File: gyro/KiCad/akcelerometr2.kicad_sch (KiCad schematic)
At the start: 5 parts, among them J2 Conn_01x04_Pin, J3 Conn_01x04_Pin, J4 Conn_01x08_Pin

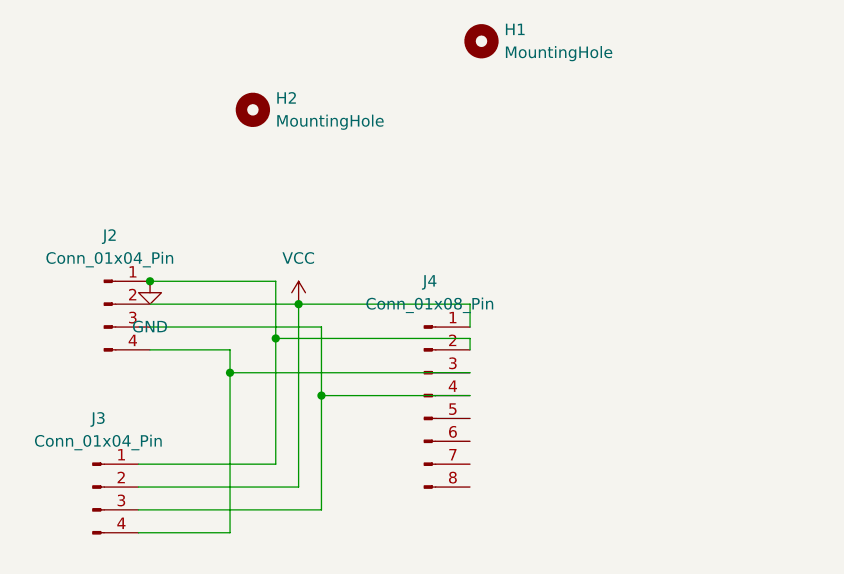
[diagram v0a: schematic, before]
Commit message: Deployed 0144617 with MkDocs version: 1.6.0
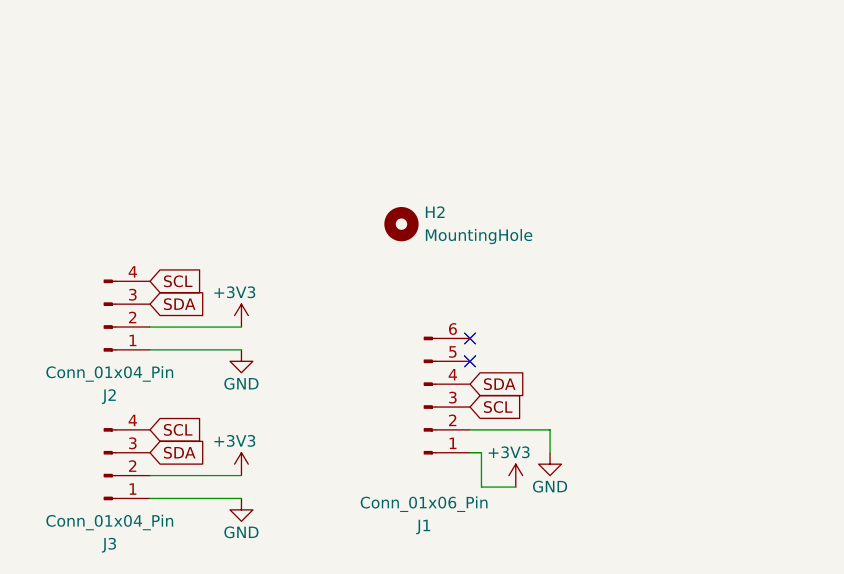
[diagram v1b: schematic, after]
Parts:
- removed H1: MountingHole, MountingHole:MountingHole_3.2mm_M3, symbol Mechanical:MountingHole
- removed J4: Conn_01x08_Pin, Connector_PinHeader_2.54mm:PinHeader_1x08_P2.54mm_Vertical, symbol Connector:Conn_01x08_Pin
- added J1: Conn_01x06_Pin, Connector_PinHeader_2.54mm:PinHeader_1x06_P2.54mm_Horizontal, symbol Connector:Conn_01x06_Pin
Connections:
- net GND: now also J1.2 (Pin_2)
- net SDA: now reaches J2.3 (Pin_3), J3.3 (Pin_3)
- net SDA: now also J1.4 (Pin_4)
- net SCL: now reaches J2.4 (Pin_4), J3.4 (Pin_4)
- net SCL: now also J1.3 (Pin_3)
- net VCC renamed +3V3
- net +3V3: now also J1.1 (Pin_1)
- no-connect marks 0 -> 2
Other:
- moved on the sheet: H2, J3

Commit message: Deployed ba208f9 with MkDocs version: 1.6.0
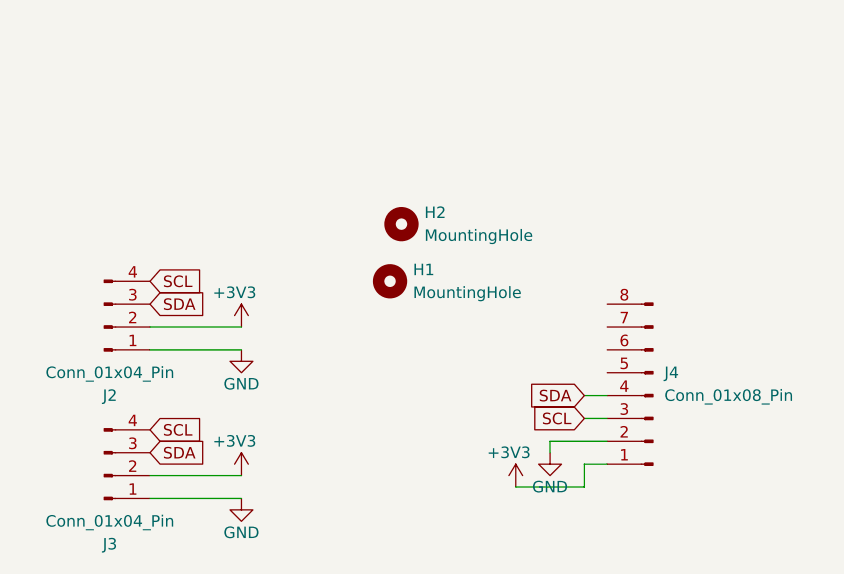
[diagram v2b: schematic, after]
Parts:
- removed J1: Conn_01x06_Pin, Connector_PinHeader_2.54mm:PinHeader_1x06_P2.54mm_Horizontal, symbol Connector:Conn_01x06_Pin
- added H1: MountingHole, MountingHole:MountingHole_3.2mm_M3, symbol Mechanical:MountingHole
- added J4: Conn_01x08_Pin, Connector_PinHeader_2.54mm:PinHeader_1x08_P2.54mm_Horizontal, symbol Connector:Conn_01x08_Pin
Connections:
- net +3V3: now also J4.1 (Pin_1)
- net GND: now also J4.2 (Pin_2)
- net SCL: now also J4.3 (Pin_3)
- net SDA: now also J4.4 (Pin_4)
- no-connect marks 2 -> 0
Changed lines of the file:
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@@
 	(generator_version "9.0")
 	(paper "A4")
-	(no_connect
-		(at 152.4 72.39)
-	)
-	(no_connect
-		(at 152.4 69.85)
-	)
 	(wire
 		(pts
@@
 	(wire
 		(pts
-			(xy 153.67 86.36) (xy 157.48 86.36)
-		)
-		(stroke
-			(width 0)
-			(type default)
-		)
-	)
-	(wire
-		(pts
-			(xy 153.67 82.55) (xy 152.4 82.55)
+			(xy 165.1 76.2) (xy 167.64 76.2)
+		)
+		(stroke
+			(width 0)
+			(type default)
+		)
+	)
+	(wire
+		(pts
+			(xy 165.1 86.36) (xy 157.48 86.36)
+		)
+		(stroke
+			(width 0)
+			(type default)
+		)
+	)
+	(wire
+		(pts
+			(xy 167.64 83.82) (xy 165.1 83.82)
+		)
+		(stroke
+			(width 0)
+			(type default)
+		)
+	)
+	(wire
+		(pts
+			(xy 165.1 78.74) (xy 167.64 78.74)
 		)
 		(stroke
@@
 	(wire
 		(pts
+			(xy 161.29 81.28) (xy 161.29 82.55)
+		)
+		(stroke
+			(width 0)
+			(type default)
+		)
+	)
+	(wire
+		(pts
 			(xy 116.84 68.58) (xy 127 68.58)
 		)
@@
 	(wire
 		(pts
-			(xy 153.67 86.36) (xy 153.67 82.55)
-		)
-		(stroke
-			(width 0)
-			(type default)
-		)
-	)
-	(wire
-		(pts
-			(xy 152.4 80.01) (xy 161.29 80.01)
-		)
-		(stroke
-			(width 0)
-			(type default)
-		)
-	)
-	(wire
-		(pts
-			(xy 161.29 80.01) (xy 161.29 82.55)
+			(xy 167.64 81.28) (xy 161.29 81.28)
+		)
+		(stroke
+			(width 0)
+			(type default)
+		)
+	)
+	(wire
+		(pts
+			(xy 165.1 83.82) (xy 165.1 86.36)
 		)
 		(stroke
@@
 	(global_label "SCL"
 		(shape input)
-		(at 152.4 77.47 0)
+		(at 165.1 78.74 180)
 		(fields_autoplaced yes)
 		(effects
@@
 				(size 1.27 1.27)
 			)
-			(justify left)
+			(justify right)
 		)
 		(property "Intersheetrefs" "${INTERSHEET_REFS}"
-			(at 158.8928 77.47 0)
-			(effects
-				(font
-					(size 1.27 1.27)
-				)
-				(justify left)
+			(at 158.6072 78.74 0)
+			(effects
+				(font
+					(size 1.27 1.27)
+				)
+				(justify right)
 				(hide yes)
 			)
@@
 	(global_label "SDA"
 		(shape input)
-		(at 152.4 74.93 0)
+		(at 165.1 76.2 180)
 		(fields_autoplaced yes)
 		(effects
@@
 				(size 1.27 1.27)
 			)
-			(justify left)
+			(justify right)
 		)
 		(property "Intersheetrefs" "${INTERSHEET_REFS}"
-			(at 158.9533 74.93 0)
-			(effects
-				(font
-					(size 1.27 1.27)
-				)
-				(justify left)
+			(at 158.5467 76.2 0)
+			(effects
+				(font
+					(size 1.27 1.27)
+				)
+				(justify right)
 				(hide yes)
 			)
@@
 	)
 	(symbol
+		(lib_id "Connector:Conn_01x08_Pin")
+		(at 172.72 76.2 180)
+		(unit 1)
+		(exclude_from_sim no)
+		(in_bom yes)
+		(on_board yes)
+		(dnp no)
+		(fields_autoplaced yes)
+		(property "Reference" "J4"
+			(at 173.99 73.6599 0)
+			(effects
+				(font
+					(size 1.27 1.27)
+				)
+				(justify right)
+			)
+		)
+		(property "Value" "Conn_01x08_Pin"
+			(at 173.99 76.1999 0)
+			(effects
+				(font
+					(size 1.27 1.27)
+				)
+				(justify right)
+			)
+		)
+		(property "Footprint" "Connector_PinHeader_2.54mm:PinHeader_1x08_P2.54mm_Horizontal"
+			(at 172.72 76.2 0)
+			(effects
+				(font
+					(size 1.27 1.27)
+				)
+				(hide yes)
+			)
+		)
+		(property "Datasheet" "~"
+			(at 172.72 76.2 0)
+			(effects
+				(font
+					(size 1.27 1.27)
+				)
+				(hide yes)
+			)
+		)
+		(property "Description" "Generic connector, single row, 01x08, script generated"
+			(at 172.72 76.2 0)
+			(effects
+				(font
+					(size 1.27 1.27)
+				)
+				(hide yes)
+			)
+		)
+		(pin "4"
+		)
+		(pin "3"
+		)
+		(pin "1"
+		)
+		(pin "2"
+		)
+		(pin "5"
+		)
+		(pin "6"
+		)
+		(pin "7"
+		)
+		(pin "8"
+		)
+		(instances
+			(project ""
+				(path "/3ee8cf12-798b-4a99-8d39-0f2ac3c6d2d6"
+					(reference "J4")
+					(unit 1)
+				)
+			)
+		)
+	)
+	(symbol
+		(lib_id "Mechanical:MountingHole")
+		(at 143.51 63.5 0)
+		(unit 1)
+		(exclude_from_sim no)
+		(in_bom no)
+		(on_board yes)
+		(dnp no)
+		(fields_autoplaced yes)
+		(property "Reference" "H1"
+			(at 146.05 62.2299 0)
+			(effects
+				(font
+					(size 1.27 1.27)
+				)
+				(justify left)
+			)
+		)
+		(property "Value" "MountingHole"
+			(at 146.05 64.7699 0)
+			(effects
+				(font
+					(size 1.27 1.27)
+				)
+				(justify left)
+			)
+		)
+		(property "Footprint" "MountingHole:MountingHole_3.2mm_M3"
+			(at 143.51 63.5 0)
+			(effects
+				(font
+					(size 1.27 1.27)
+				)
+				(hide yes)
+			)
+		)
+		(property "Datasheet" "~"
+			(at 143.51 63.5 0)
+			(effects
+				(font
+					(size 1.27 1.27)
+				)
+				(hide yes)
+			)
+		)
+		(property "Description" "Mounting Hole without connection"
+			(at 143.51 63.5 0)
+			(effects
+				(font
+					(size 1.27 1.27)
+				)
+				(hide yes)
+			)
+		)
+		(instances
+			(project "akcelerometr2"
+				(path "/3ee8cf12-798b-4a99-8d39-0f2ac3c6d2d6"
+					(reference "H1")
+					(unit 1)
+				)
+			)
+		)
+	)
+	(symbol
 		(lib_id "power:+3V3")
 		(at 127 85.09 0)
@@
 					(unit 1)
 				)
-			)
-		)
-	)
-	(symbol
-		(lib_id "Connector:Conn_01x06_Pin")
-		(at 147.32 77.47 0)
-		(mirror x)
-		(unit 1)
-		(exclude_from_sim no)
-		(in_bom yes)
-		(on_board yes)
-		(dnp no)
-		(property "Reference" "J1"
-			(at 147.32 90.678 0)
-			(effects
-				(font
-					(size 1.27 1.27)
-				)
-			)
-		)
-		(property "Value" "Conn_01x06_Pin"
-			(at 147.32 88.138 0)
-			(effects
-				(font
-					(size 1.27 1.27)
-				)
-			)
-		)
-		(property "Footprint" "Connector_PinHeader_2.54mm:PinHeader_1x06_P2.54mm_Horizontal"
-			(at 147.32 77.47 0)
-			(effects
-				(font
-					(size 1.27 1.27)
-				)
-				(hide yes)
-			)
-		)
-		(property "Datasheet" "~"
-			(at 147.32 77.47 0)
-			(effects
-				(font
-					(size 1.27 1.27)
-				)
-				(hide yes)
-			)
-		)
-		(property "Description" "Generic connector, single row, 01x06, script generated"
-			(at 147.32 77.47 0)
-			(effects
-				(font
-					(size 1.27 1.27)
-				)
-				(hide yes)
-			)
-		)
-		(pin "6"
-		)
-		(pin "4"
-		)
-		(pin "1"
-		)
-		(pin "5"
-		)
-		(pin "3"
-		)
-		(pin "2"
-		)
-		(instances
-			(project "akcelerometr2"
-				(path "/3ee8cf12-798b-4a99-8d39-0f2ac3c6d2d6"
-					(reference "J1")
-					(unit 1)
-				)
